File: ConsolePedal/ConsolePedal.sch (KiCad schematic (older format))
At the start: 1 part, among them U1 N64-Cartridge

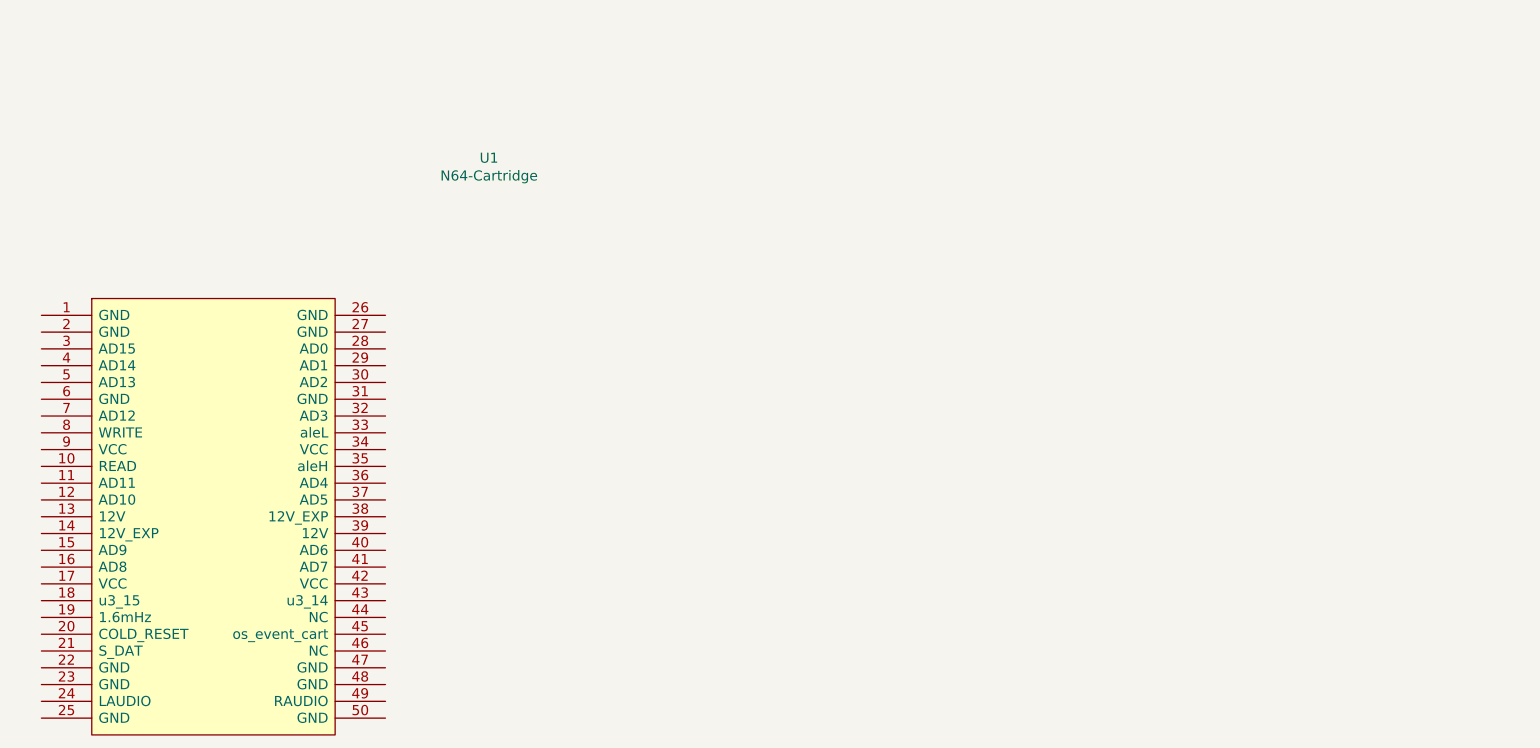
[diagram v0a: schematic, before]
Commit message: Finished schematic
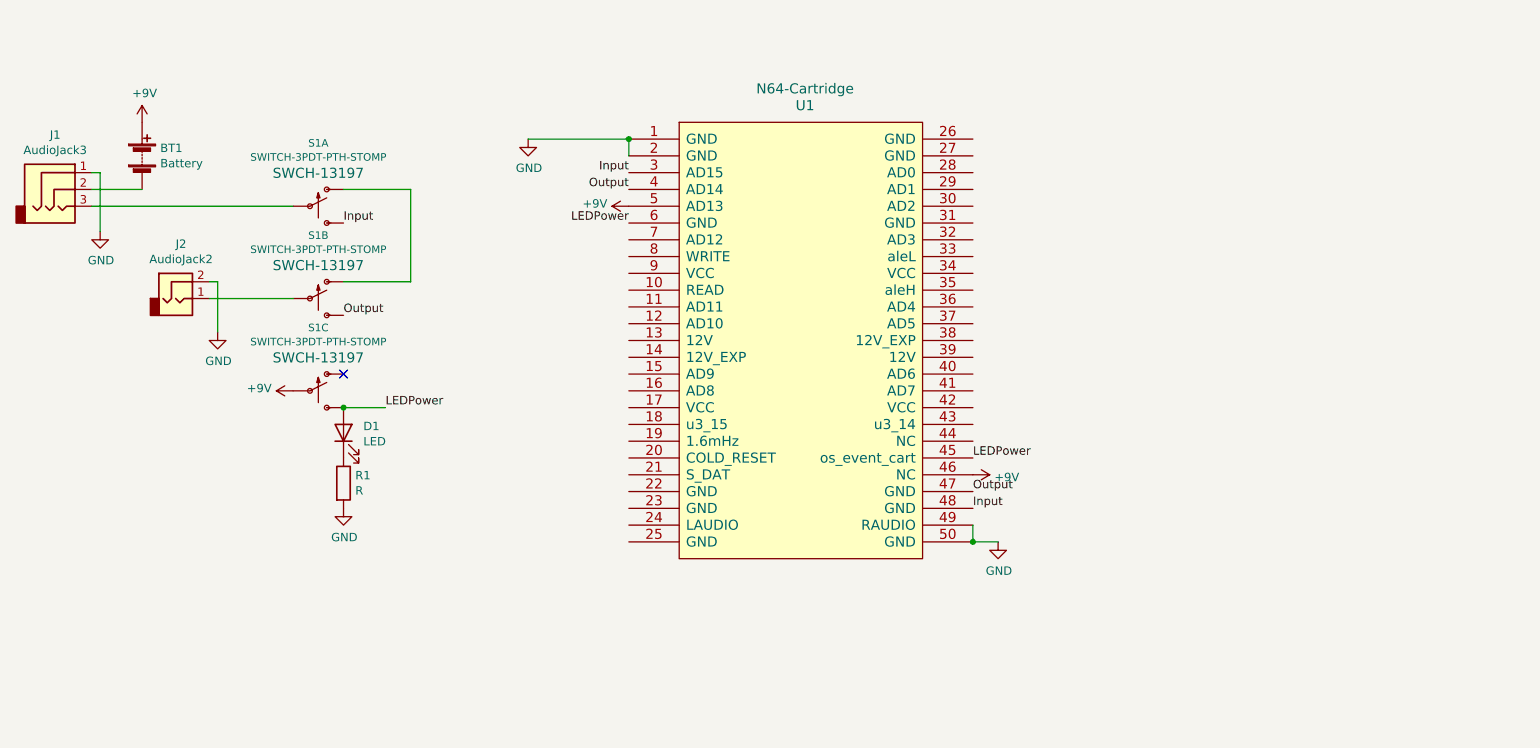
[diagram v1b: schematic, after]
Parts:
- added BT1: Battery, symbol Device:Battery
- added D1: LED, LED_THT:LED_D5.0mm, symbol Device:LED
- added J1: AudioJack3, Connector_PinSocket_2.54mm:PinSocket_1x03_P2.54mm_Vertical, symbol audioJacks:AudioJack3
- added J2: AudioJack2, Connector_PinSocket_2.54mm:PinSocket_1x02_P2.54mm_Vertical, symbol audioJacks:AudioJack2
- added R1: R, Resistor_THT:R_Axial_DIN0207_L6.3mm_D2.5mm_P10.16mm_Horizontal, symbol Device:R
- added S1: SWITCH-3PDT-PTH-STOMP, MuffPi:STOMP_SWITCH_3PDT, symbol SparkFun-Switches:SWITCH-3PDT-PTH-STOMP
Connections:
- net GND: now reaches U1.1 (GND)
- net GND: now also U1.2 (GND), U1.49 (RAUDIO), U1.50 (GND), J1.1, J2.2, R1.2
- net Input: now reaches U1.3 (AD15)
- net Input: now also U1.48 (GND), S1.P$3 (S)
- net Output: now reaches U1.4 (AD14)
- net Output: now also U1.47 (GND), S1.P$6 (S)
- net LEDPower: now reaches U1.45 (os_event_cart)
- net LEDPower: now also U1.6 (GND), D1.2 (A), S1.P$9 (S)
- net +9V: now reaches U1.46 (NC)
- net +9V: now also U1.5 (AD13), BT1.1 (+), S1.P$8 (P)
- new net: J2.1, S1.P$5 (P)
- new net: BT1.2 (-), J1.2
- new net: J1.3, S1.P$2 (P)
- new net: S1.P$1 (O), S1.P$4 (O)
- new net: D1.1 (K), R1.1
- no-connect marks 0 -> 1
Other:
- moved on the sheet: U1
